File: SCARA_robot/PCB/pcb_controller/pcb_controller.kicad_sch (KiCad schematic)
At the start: 50 parts, among them J1 Barrel_Jack_Switch, J10 interface, J11 Conn_01x07_Socket, J12 Encoder_A, J13 Encoder_B, J14 Encoder_C, J15 Conn_01x04_Pin_STEPPER_B, J16 Conn_01x04_Pin_STEPPER_C, J2 Conn_01x04_Pin_STEPPER_A, J3 interface, J4 power, J5 Conn_01x07_Socket, J6 power, J7 interface, J8 Conn_01x07_Socket, J9 power, SW1 Microstep mode, SW2 Microstep mode, SW3 Microstep mode, U1 LM7805CT, U2 ESP32-DEVKIT-V1, U3 PCA9548A, U4 LD1117S33TR_SOT223

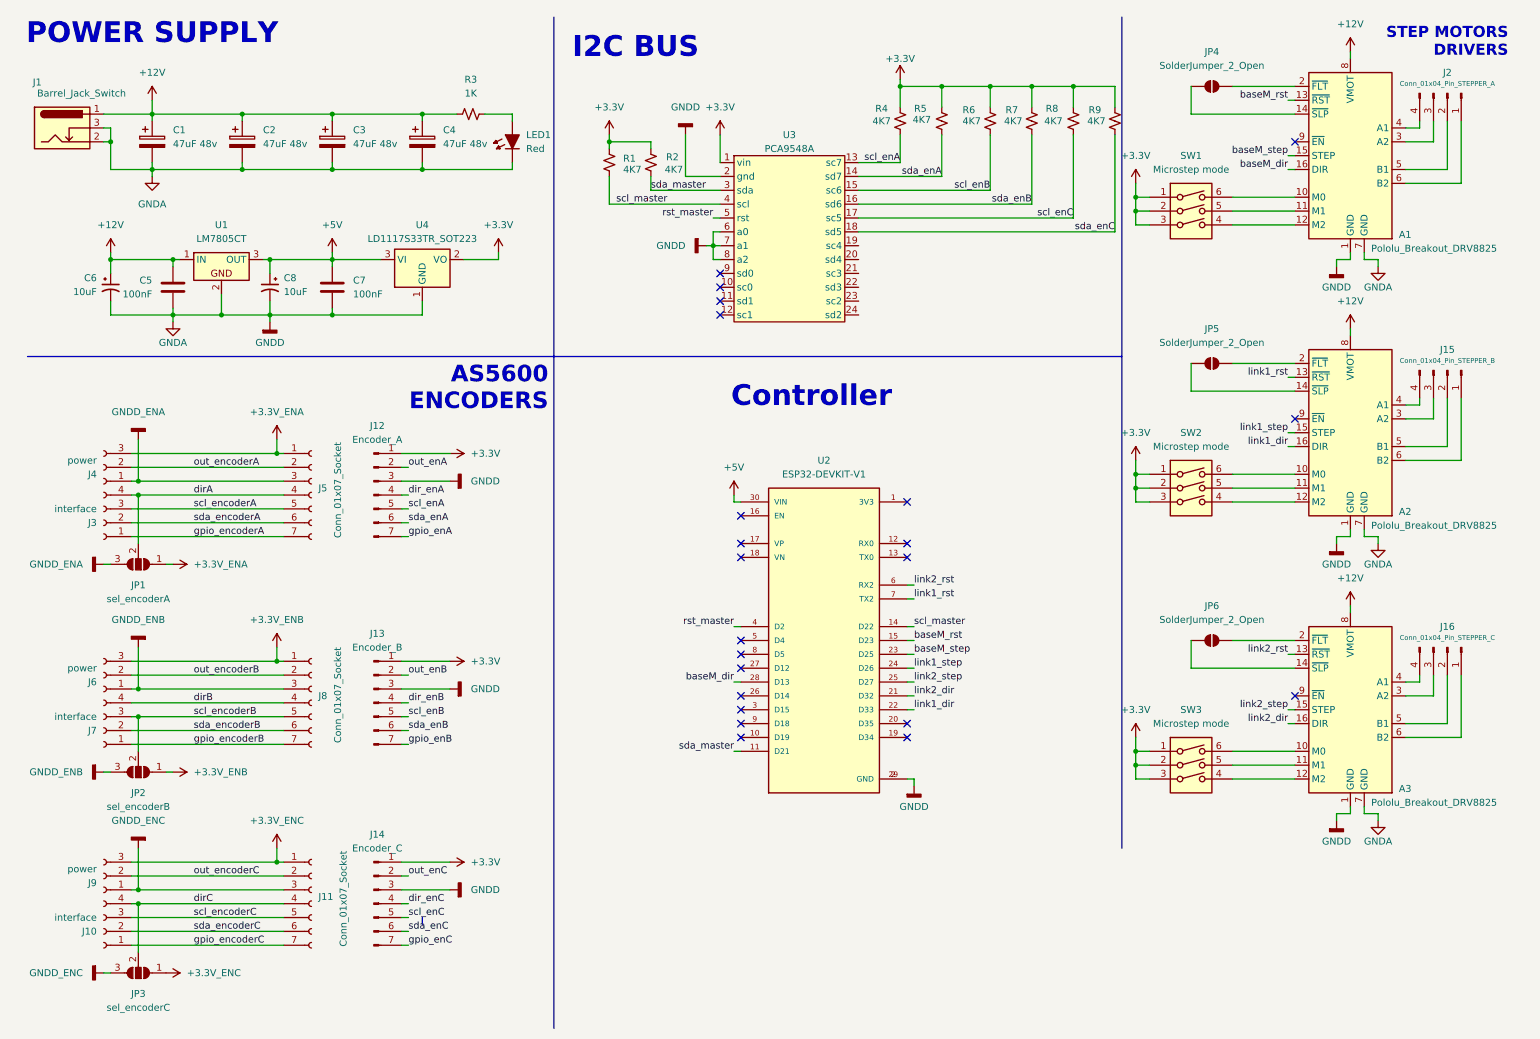
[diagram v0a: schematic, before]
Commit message: pcb designed phase 1
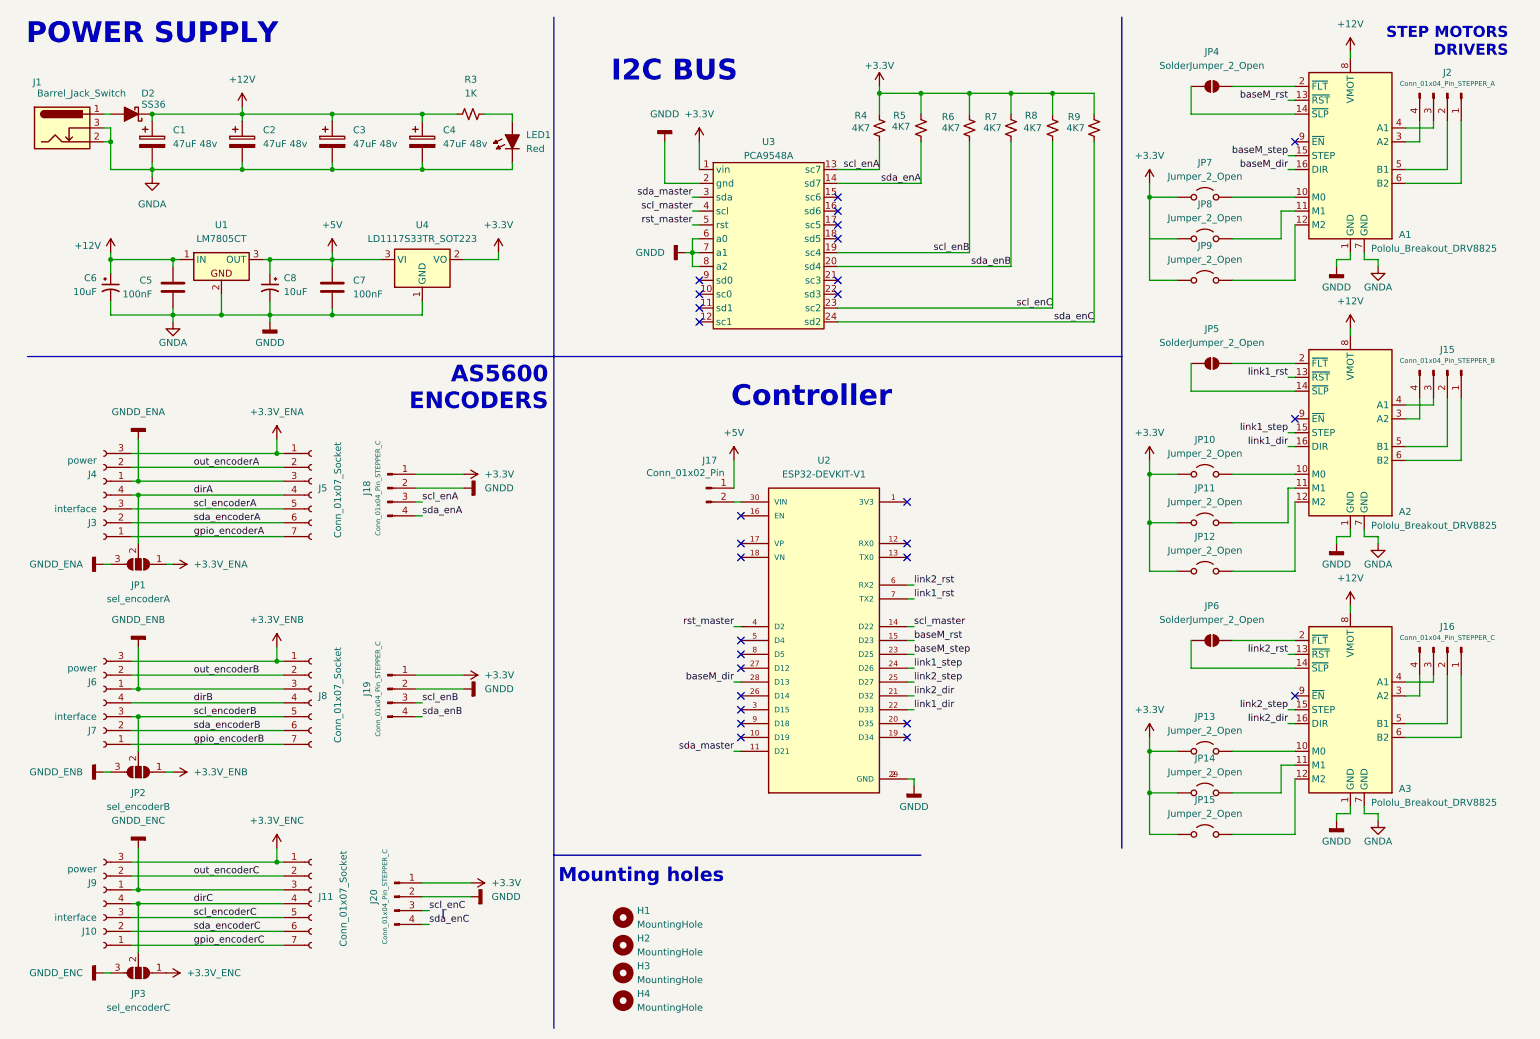
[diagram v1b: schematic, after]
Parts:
- removed J12: Encoder_A, Connector_JST:JST_XH_B7B-XH-AM_1x07_P2.50mm_Vertical, symbol Connector:Conn_01x07_Pin
- removed J13: Encoder_B, Connector_JST:JST_XH_B7B-XH-AM_1x07_P2.50mm_Vertical, symbol Connector:Conn_01x07_Pin
- removed J14: Encoder_C, Connector_JST:JST_XH_B7B-XH-AM_1x07_P2.50mm_Vertical, symbol Connector:Conn_01x07_Pin
- removed R1, R2: 4K7, PCM_Resistor_THT_AKL:R_Axial_DIN0204_L3.6mm_D1.6mm_P5.08mm_Horizontal, symbol Device:R_Small_US
- removed SW1, SW2, SW3: Microstep mode, Button_Switch_THT:SW_DIP_SPSTx03_Slide_9.78x9.8mm_W7.62mm_P2.54mm, symbol Switch:SW_DIP_x03
- added D2: SS36, Diode_SMD:D_2114_3652Metric_Pad1.85x3.75mm_HandSolder, symbol PCM_Diode_Schottky_AKL:SS36
- added H1, H2, H3, H4: MountingHole, MountingHole:MountingHole_3.2mm_M3_ISO14580, symbol Mechanical:MountingHole
- added J17: Conn_01x02_Pin, Connector_PinSocket_2.54mm:PinSocket_1x02_P2.54mm_Vertical, symbol Connector:Conn_01x02_Pin
- added J18, J19, J20: Conn_01x04_Pin_STEPPER_C, Connector_JST:JST_XH_B4B-XH-AM_1x04_P2.50mm_Vertical, symbol Connector:Conn_01x04_Pin
- added JP10, JP11, JP12, JP13, JP14, JP15, JP7, JP8, JP9: Jumper_2_Open, PCM_Jumper_AKL:Jumper_P2.54mm_D0.7mm, symbol Jumper:Jumper_2_Open
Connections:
- net +12V: now also D2.1 (K); no longer J1.1
- net +3.3V: now also J18.1 (Pin_1), J19.1 (Pin_1), J20.1 (Pin_1), JP10.1 (A), JP11.1 (A), JP12.1 (A), JP13.1 (A), JP14.1 (A), JP15.1 (A), JP7.1 (A), JP9.1 (A)
- net +5V: now also J17.1 (Pin_1); no longer U2.30 (VIN)
- net GNDA: now also J18.2 (Pin_2), J19.2 (Pin_2), J20.2 (Pin_2)
- net scl_enA: now also J18.3 (Pin_3)
- net scl_enB: now also U3.19 (sc4), J19.3 (Pin_3); no longer U3.15 (sc6)
- net scl_enC: now also U3.23 (sc2), J20.3 (Pin_3); no longer U3.17 (sc5)
- net sda_enA: now also J18.4 (Pin_4)
- net sda_enB: now also U3.20 (sd4), J19.4 (Pin_4); no longer U3.16 (sd6)
- net sda_enC: now also U3.24 (sd2), J20.4 (Pin_4); no longer U3.18 (sd5)
- net at A3.12 (M2): now also JP15.2 (B)
- net at A3.11 (M1): now also JP14.2 (B)
- net at A3.10 (M0): now also JP13.2 (B)
- net at J2.3 (Pin_3): now also A1.4 (A1); no longer A1.3 (A2)
- net at J2.4 (Pin_4): now also A1.3 (A2); no longer A1.4 (A1)
- net at A2.12 (M2): now also JP12.2 (B)
- net at A2.11 (M1): now also JP11.2 (B)
- net at A2.10 (M0): now also JP10.2 (B)
- net at J15.3 (Pin_3): now also A2.4 (A1); no longer A2.3 (A2)
- net at J15.4 (Pin_4): now also A2.3 (A2); no longer A2.4 (A1)
- net at A1.12 (M2): now also JP9.2 (B)
- net at A1.11 (M1): now also JP8.2 (B)
- net at A1.10 (M0): now also JP7.2 (B)
- net at J16.3 (Pin_3): now also A3.4 (A1); no longer A3.3 (A2)
- net at J16.4 (Pin_4): now also A3.3 (A2); no longer A3.4 (A1)
- new net: D2.2 (A), J1.1
- new net: J17.2 (Pin_2), U2.30 (VIN)
- no-connect marks 22 -> 28
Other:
- note added: "Mounting holes"
- moved on the sheet: R4, R5, R6, R7, R8, R9, U3
